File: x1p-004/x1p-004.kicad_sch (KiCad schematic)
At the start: 14 parts, among them U1 AD24C02, U2 SN74LVC1T45DBVR, U3 SN74LVC1T45DBVR, U4 2060-452/998-404, U5 2060-452/998-404

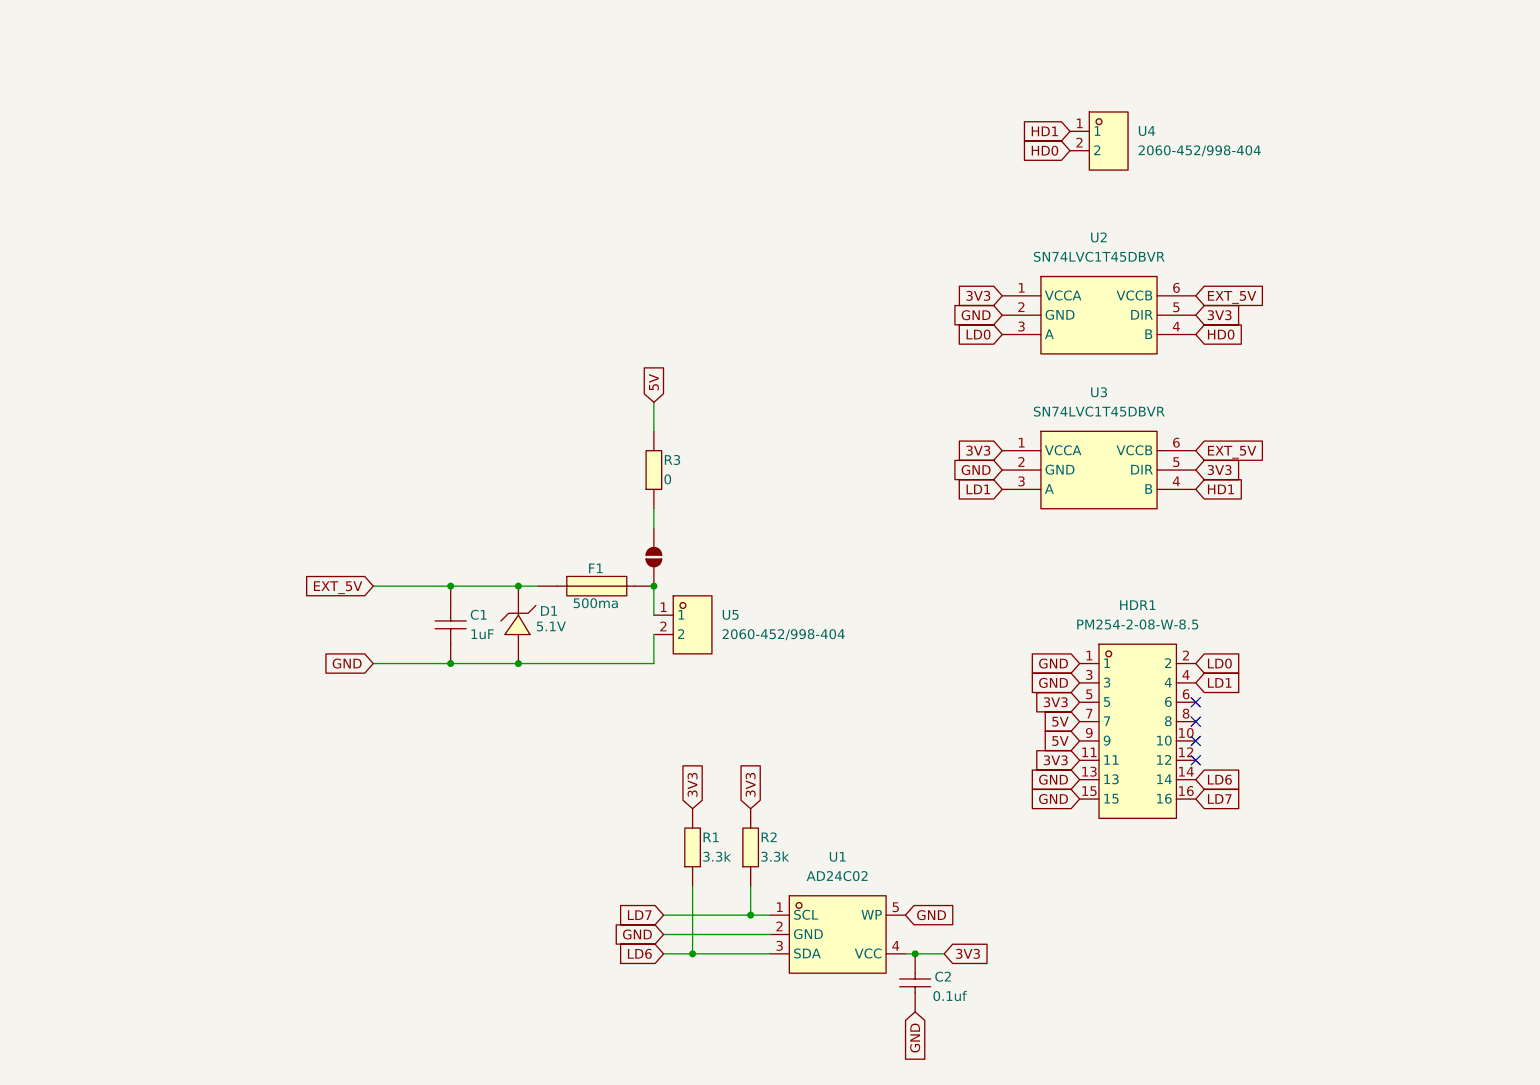
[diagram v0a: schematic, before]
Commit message: changes round 2
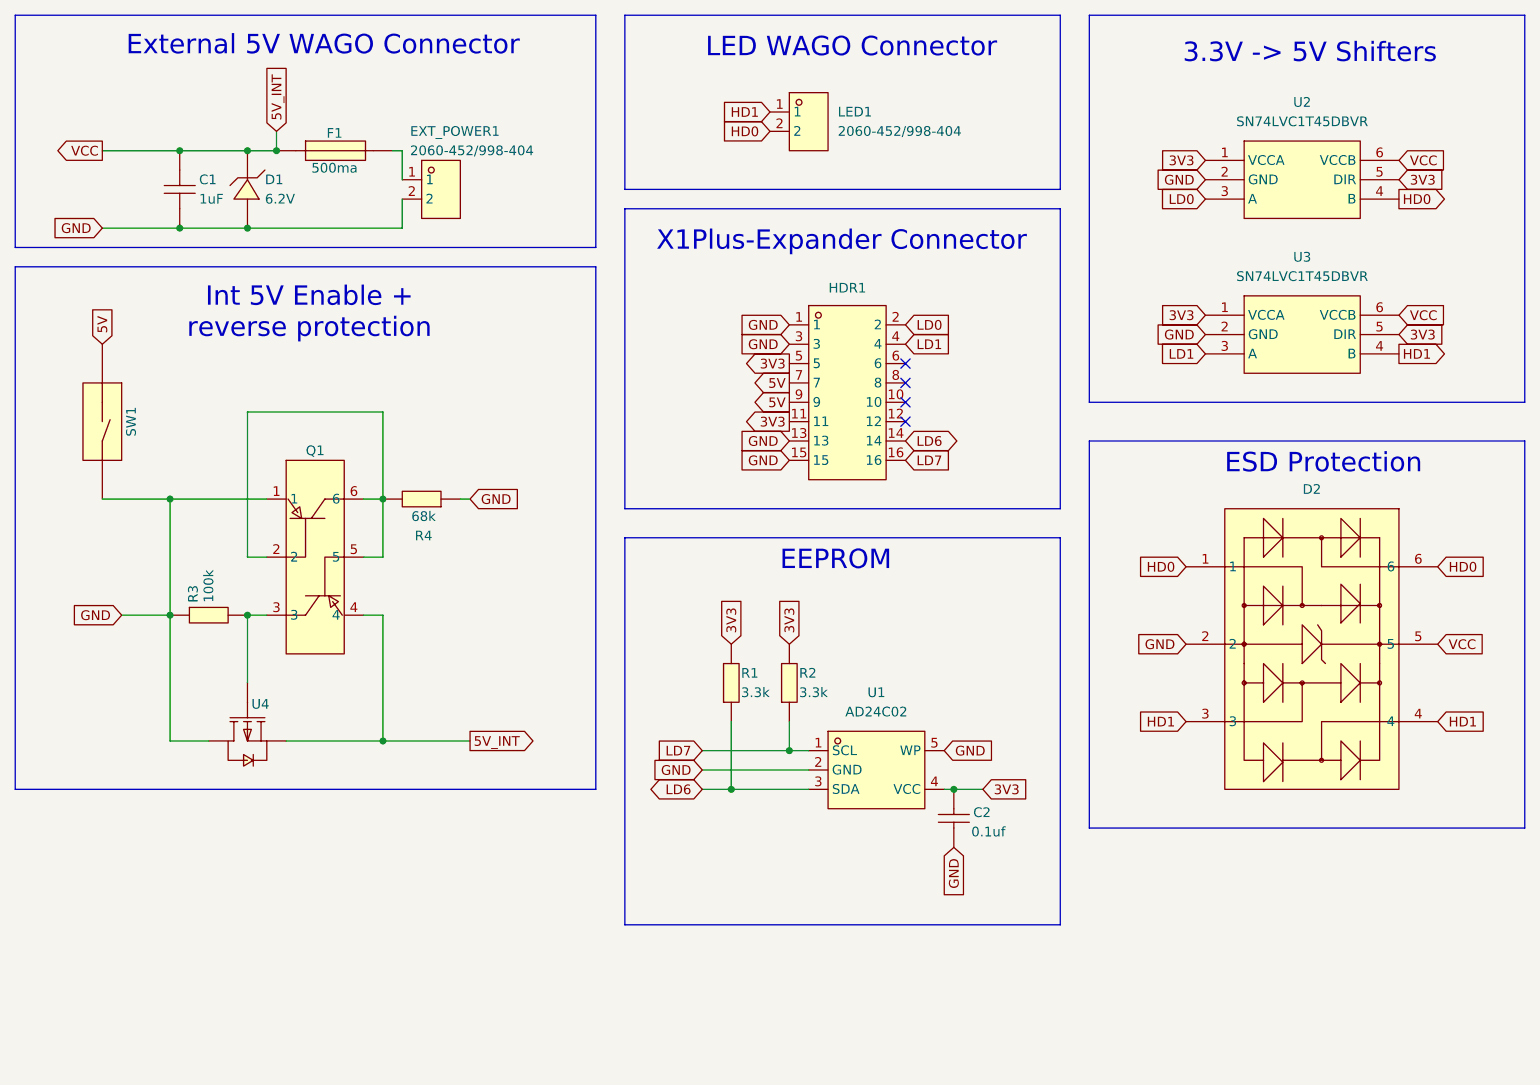
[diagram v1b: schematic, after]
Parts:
- removed D1: 5.1V, lcsc:SOD-123_L2.8-W1.8-LS3.7-RD, symbol lcsc:MMSZ5231B-7-F
- removed JP1: SolderJumper_2_Open, Jumper:SolderJumper-2_P1.3mm_Open_RoundedPad1.0x1.5mm, symbol Jumper:SolderJumper_2_Open
- removed R3: 0, lcsc:R0603, symbol lcsc:0603WAF0000T5E
- removed U5: 2060-452/998-404, lcsc:CONN-SMD_2060-452, symbol lcsc:2060-452_998-404
- added D1: 6.2V, x1p-004:SOD-123_L2.8-W1.8-LS3.7-RD, symbol x1p-004:MMSZ5234BT1G
- added D2: SRV05-4.TCT_C2687126, x1p-004:SOT-23-6_L2.9-W1.6-P0.95-LS2.8-BL, symbol x1p-004:SRV05-4.TCT_C2687126
- added EXT_POWER1: 2060-452/998-404, x1p-004:CONN-SMD_2060-452, symbol lcsc:2060-452_998-404
- added Q1: BC857BS,115, x1p-004:SOT-363_L2.0-W1.3-P0.65-LS2.1-TL, symbol lcsc:BC857BS,115
- added R3: 100k, x1p-004:R0402, symbol lcsc:0402WGF1003TCE
- added R4: 68k, x1p-004:R0402, symbol lcsc:0402WGF6802TCE
- added SW1: DSIC01THGET, x1p-004:SW-TH_DSIC01THGET, symbol x1p-004:DSIC01THGET
- added U4: SI2301-ZE, x1p-004:SOT-23-3_L2.9-W1.3-P1.90-LS2.4-BR, symbol lcsc:SI2301-ZE
- C1: footprint lcsc:C0603 -> x1p-004:C0603
- C2: footprint lcsc:C0402 -> x1p-004:C0402
- HDR1: footprint lcsc:HDR-TH_16P-P2.54-H-F-R2-C8-W8.5 -> x1p-004:HDR-TH_16P-P2.54-H-F-R2-C8-W8.5
- LED1: renamed from U4; footprint lcsc:CONN-SMD_2060-452 -> x1p-004:CONN-SMD_2060-452
- R1, R2: footprint lcsc:R0402 -> x1p-004:R0402
- U1: footprint lcsc:SOT-23-5_L2.9-W1.6-P0.95-LS2.8-BL -> x1p-004:SOT-23-5_L2.9-W1.6-P0.95-LS2.8-BL
- U2, U3: footprint lcsc:SOT-23-6_L2.9-W1.6-P0.95-LS2.8-BR -> x1p-004:SOT-23-6_L2.9-W1.6-P0.95-LS2.8-BR
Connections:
- net 5V: now also SW1.1
- net GND: now also D1.2 (A), D2.2, EXT_POWER1.2, Q1.1, R3.1, R4.1, SW1.2, U4.3 (D)
- net HD0: now also D2.1, D2.6
- net HD1: now also D2.3, D2.4
- net at F1.2: now also EXT_POWER1.1
- net EXT_5V renamed 5V_INT
- net 5V_INT: now also D1.1 (C), D2.5, Q1.4, U4.2 (S)
- new net: Q1.3, R3.2, U4.1 (G)
- new net: Q1.2, Q1.5, Q1.6, R4.2
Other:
- note added: "3.3V -> 5V Shifters"
- note added: "EEPROM"
- note added: "ESD Protection"
- note added: "External 5V WAGO Connector"
- note added: "Int 5V Enable + reverse protection"
- note added: "LED WAGO Connector"
- note added: "X1Plus-Expander Connector"
- moved on the sheet: C2, HDR1, LED1, R1, R2, U1, U2, U3
